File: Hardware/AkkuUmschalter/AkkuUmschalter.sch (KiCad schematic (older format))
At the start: 5 parts

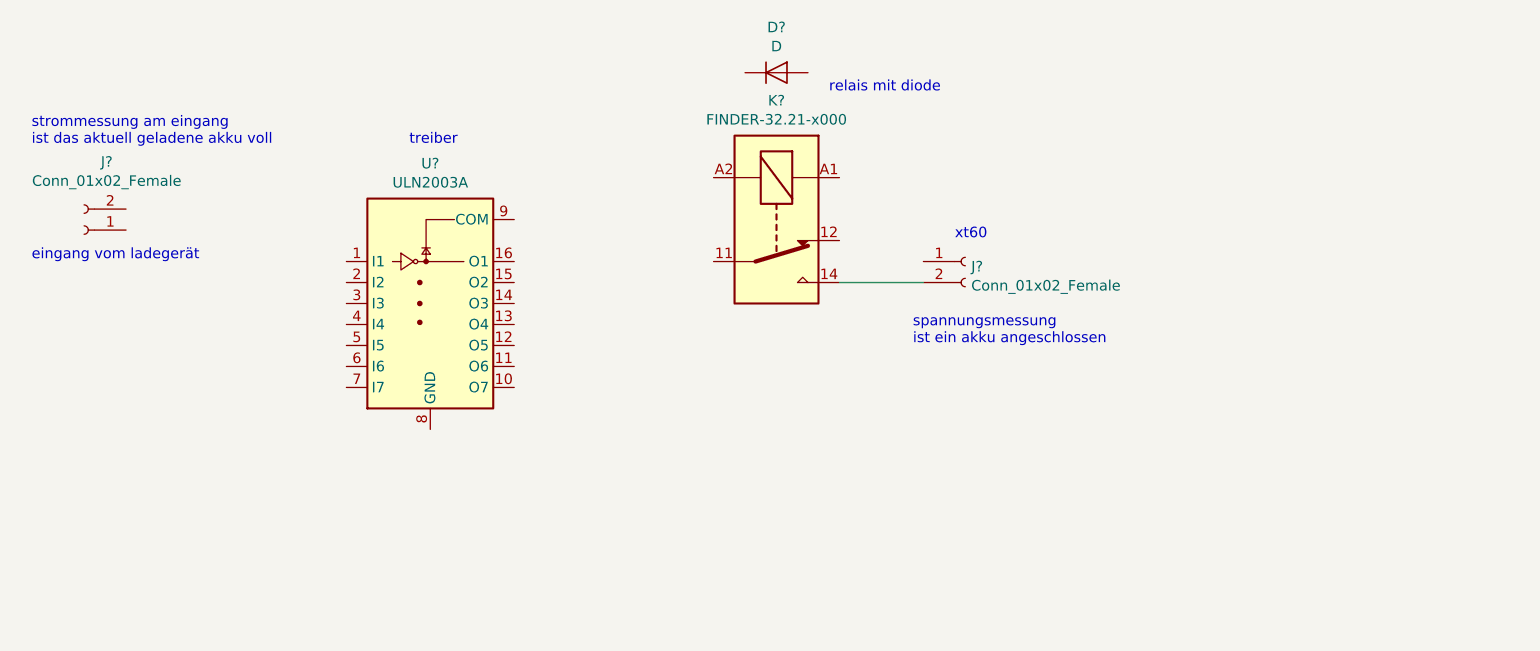
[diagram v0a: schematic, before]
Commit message: progress and voltage sensing
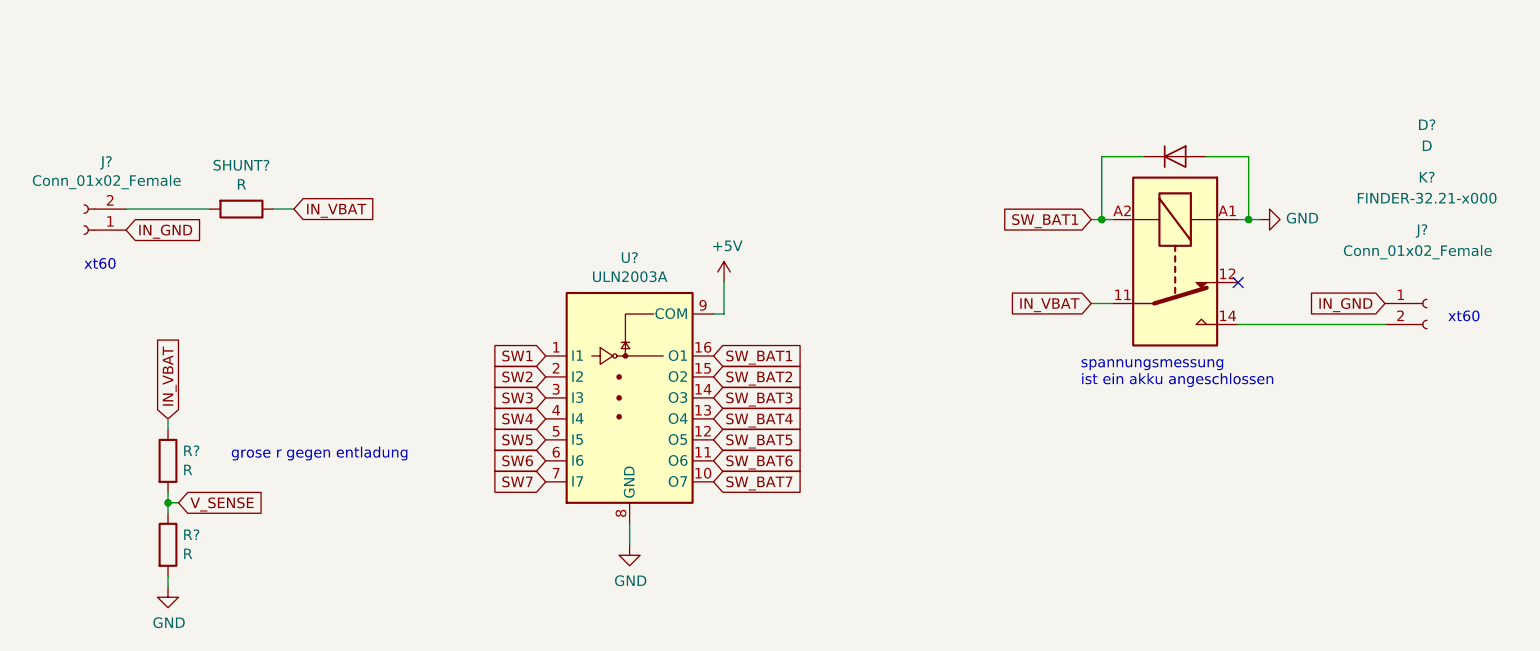
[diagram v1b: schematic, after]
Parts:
- added R? (x2), SHUNT?: R, symbol Device:R
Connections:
- net IN_VBAT: now reaches K?.11
- net IN_VBAT: now also R?.1, SHUNT?.1
- net GND: now reaches K?.A1
- net GND: now also D?.2 (A), U?.8 (GND), R?.2
- net SW_BAT1: now reaches K?.A2
- net SW_BAT1: now also D?.1 (K), U?.16 (O1)
- net IN_GND: now reaches J?.1 (Pin_1)
- net IN_GND: now also J?.1 (Pin_1)
- net SW1: now reaches U?.1 (I1)
- net SW_BAT7: now reaches U?.10 (O7)
- net SW_BAT6: now reaches U?.11 (O6)
- net SW_BAT5: now reaches U?.12 (O5)
- net SW_BAT4: now reaches U?.13 (O4)
- net SW_BAT3: now reaches U?.14 (O3)
- net SW_BAT2: now reaches U?.15 (O2)
- net SW2: now reaches U?.2 (I2)
- net SW3: now reaches U?.3 (I3)
- net SW4: now reaches U?.4 (I4)
- net SW5: now reaches U?.5 (I5)
- net SW6: now reaches U?.6 (I6)
- net SW7: now reaches U?.7 (I7)
- net +5V: now reaches U?.9 (COM)
- net at J?.2 (Pin_2): now also SHUNT?.2
- new net V_SENSE: R?.1, R?.2
- no-connect marks 0 -> 1
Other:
- note added: "grose r gegen entladung"
- note removed: "eingang vom ladegerät"
- note removed: "relais mit diode"
- note removed: "strommessung am eingang\nist das aktuell geladene akku voll"
- note removed: "treiber"
- moved on the sheet: D?, J?, K?, U?
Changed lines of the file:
@@
 L Relay:FINDER-32.21-x000 K?
 U 1 1 5E258ADA
-P 4300 1700
-F 0 "K?" V 3733 1700 50  0000 C CNN
-F 1 "FINDER-32.21-x000" V 3824 1700 50  0000 C CNN
-F 2 "" H 5570 1670 50  0001 C CNN
-F 3 "https://gfinder.findernet.com/assets/Series/355/S32EN.pdf" H 4300 1700 50  0001 C CNN
-	1    4300 1700
+P 6200 1900
+F 0 "K?" V 5800 3100 50  0000 C CNN
+F 1 "FINDER-32.21-x000" V 5900 3100 50  0000 C CNN
+F 2 "" H 7470 1870 50  0001 C CNN
+F 3 "https://gfinder.findernet.com/assets/Series/355/S32EN.pdf" H 6200 1900 50  0001 C CNN
+	1    6200 1900
 	0    1    1    0
 $EndComp
-$Comp
-L Connector:Conn_01x02_Female J?
-U 1 1 5E25A7F8
-P 5200 1900
-F 0 "J?" H 5228 1876 50  0000 L CNN
-F 1 "Conn_01x02_Female" H 5228 1785 50  0000 L CNN
-F 2 "" H 5200 1900 50  0001 C CNN
-F 3 "~" H 5200 1900 50  0001 C CNN
-	1    5200 1900
-	1    0    0    -1
-$EndComp
-Wire Wire Line
-	4600 2000 5000 2000
+Wire Wire Line
+	6500 2200 7200 2200
 $Comp
 L Transistor_Array:ULN2003A U?
 U 1 1 5E25DBBD
-P 2650 2100
-F 0 "U?" H 2650 2767 50  0000 C CNN
-F 1 "ULN2003A" H 2650 2676 50  0000 C CNN
-F 2 "" H 2700 1550 50  0001 L CNN
-F 3 "http://www.ti.com/lit/ds/symlink/uln2003a.pdf" H 2750 1900 50  0001 C CNN
-	1    2650 2100
+P 3600 2550
+F 0 "U?" H 3600 3217 50  0000 C CNN
+F 1 "ULN2003A" H 3600 3126 50  0000 C CNN
+F 2 "" H 3650 2000 50  0001 L CNN
+F 3 "http://www.ti.com/lit/ds/symlink/uln2003a.pdf" H 3700 2350 50  0001 C CNN
+	1    3600 2550
 	1    0    0    -1
 $EndComp
@@
 L Device:D D?
 U 1 1 5E25ED1E
-P 4300 1000
-F 0 "D?" H 4300 1216 50  0000 C CNN
-F 1 "D" H 4300 1125 50  0000 C CNN
-F 2 "" H 4300 1000 50  0001 C CNN
-F 3 "~" H 4300 1000 50  0001 C CNN
-	1    4300 1000
-	1    0    0    -1
-$EndComp
-Text Notes 5150 1800 0    50   ~ 0
+P 6200 1400
+F 0 "D?" H 7400 1550 50  0000 C CNN
+F 1 "D" H 7400 1450 50  0000 C CNN
+F 2 "" H 6200 1400 50  0001 C CNN
+F 3 "~" H 6200 1400 50  0001 C CNN
+	1    6200 1400
+	1    0    0    -1
+$EndComp
+Text Notes 7500 2200 0    50   ~ 0
 xt60
-Text Notes 2550 1350 0    50   ~ 0
-treiber
-Text Notes 4550 1100 0    50   ~ 0
-relais mit diode
-Text Notes 4950 2300 0    50   ~ 0
+Text Notes 5750 2500 0    50   ~ 0
 spannungsmessung\nist ein akku angeschlossen
-Text Notes 750  1350 0    50   ~ 0
-strommessung am eingang\nist das aktuell geladene akku voll
 $Comp
 L Connector:Conn_01x02_Female J?
@@
 	-1   0    0    1
 $EndComp
-Text Notes 750  1900 0    50   ~ 0
-eingang vom ladegerät
+$Comp
+L power:+5V #PWR?
+U 1 1 5E274D46
+P 4050 2000
+F 0 "#PWR?" H 4050 1850 50  0001 C CNN
+F 1 "+5V" H 4065 2173 50  0000 C CNN
+F 2 "" H 4050 2000 50  0001 C CNN
+F 3 "" H 4050 2000 50  0001 C CNN
+	1    4050 2000
+	1    0    0    -1
+$EndComp
+$Comp
+L power:GND #PWR?
+U 1 1 5E275841
+P 3600 3250
+F 0 "#PWR?" H 3600 3000 50  0001 C CNN
+F 1 "GND" H 3605 3077 50  0000 C CNN
+F 2 "" H 3600 3250 50  0001 C CNN
+F 3 "" H 3600 3250 50  0001 C CNN
+	1    3600 3250
+	1    0    0    -1
+$EndComp
+$Comp
+L power:GND #PWR?
+U 1 1 5E27671A
+P 6600 1700
+F 0 "#PWR?" H 6600 1450 50  0001 C CNN
+F 1 "GND" V 6605 1572 50  0000 R CNN
+F 2 "" H 6600 1700 50  0001 C CNN
+F 3 "" H 6600 1700 50  0001 C CNN
+	1    6600 1700
+	0    -1   -1   0
+$EndComp
+Wire Wire Line
+	6600 1700 6550 1700
+Wire Wire Line
+	6550 1700 6550 1400
+Wire Wire Line
+	6550 1400 6350 1400
+Connection ~ 6550 1700
+Wire Wire Line
+	6550 1700 6500 1700
+Wire Wire Line
+	6050 1400 5850 1400
+Wire Wire Line
+	5850 1400 5850 1700
+Wire Wire Line
+	5850 1700 5900 1700
+NoConn ~ 6500 2000
+Wire Wire Line
+	3600 3250 3600 3150
+Wire Wire Line
+	4000 2150 4050 2150
+Wire Wire Line
+	4050 2150 4050 2000
+Text GLabel 4000 2350 2    50   Input ~ 0
+SW_BAT1
+Text GLabel 4000 2450 2    50   Input ~ 0
+SW_BAT2
+Text GLabel 4000 2550 2    50   Input ~ 0
+SW_BAT3
+Text GLabel 4000 2650 2    50   Input ~ 0
+SW_BAT4
+Text GLabel 4000 2750 2    50   Input ~ 0
+SW_BAT5
+Text GLabel 4000 2850 2    50   Input ~ 0
+SW_BAT6
+Text GLabel 4000 2950 2    50   Input ~ 0
+SW_BAT7
+Text GLabel 5800 1700 0    50   Input ~ 0
+SW_BAT1
+Wire Wire Line
+	5850 1700 5800 1700
+Connection ~ 5850 1700
+$Comp
+L Connector:Conn_01x02_Female J?
+U 1 1 5E25A7F8
+P 7400 2100
+F 0 "J?" H 7350 2450 50  0000 L CNN
+F 1 "Conn_01x02_Female" H 7000 2350 50  0000 L CNN
+F 2 "" H 7400 2100 50  0001 C CNN
+F 3 "~" H 7400 2100 50  0001 C CNN
+	1    7400 2100
+	1    0    0    -1
+$EndComp
+$Comp
+L Device:R SHUNT?
+U 1 1 5E27EAD8
+P 1750 1650
+F 0 "SHUNT?" V 1543 1650 50  0000 C CNN
+F 1 "R" V 1634 1650 50  0000 C CNN
+F 2 "" V 1680 1650 50  0001 C CNN
+F 3 "~" H 1750 1650 50  0001 C CNN
+	1    1750 1650
+	0    1    1    0
+$EndComp
+Text Notes 1000 1950 0    50   ~ 0
+xt60
+Wire Wire Line
+	1200 1650 1600 1650
+Text GLabel 1200 1750 2    50   Input ~ 0
+IN_GND
+Text GLabel 7200 2100 0    50   Input ~ 0
+IN_GND
+Text GLabel 2000 1650 2    50   Input ~ 0
+IN_VBAT
+Wire Wire Line
+	2000 1650 1900 1650
+Text GLabel 5800 2100 0    50   Input ~ 0
+IN_VBAT
+Wire Wire Line
+	5800 2100 5900 2100
+Text GLabel 3200 2350 0    50   Input ~ 0
+SW1
+Text GLabel 3200 2450 0    50   Input ~ 0
+SW2
+Text GLabel 3200 2550 0    50   Input ~ 0
+SW3
+Text GLabel 3200 2650 0    50   Input ~ 0
+SW4
+Text GLabel 3200 2750 0    50   Input ~ 0
+SW5
+Text GLabel 3200 2850 0    50   Input ~ 0
+SW6
+Text GLabel 3200 2950 0    50   Input ~ 0
+SW7
+$Comp
+L Device:R R?
+U 1 1 5E281E20
+P 1400 2850
+F 0 "R?" H 1470 2896 50  0000 L CNN
+F 1 "R" H 1470 2805 50  0000 L CNN
+F 2 "" V 1330 2850 50  0001 C CNN
+F 3 "~" H 1400 2850 50  0001 C CNN
+	1    1400 2850
+	1    0    0    -1
+$EndComp
+$Comp
+L Device:R R?
+U 1 1 5E2827A1
+P 1400 3250
+F 0 "R?" H 1470 3296 50  0000 L CNN
+F 1 "R" H 1470 3205 50  0000 L CNN
+F 2 "" V 1330 3250 50  0001 C CNN
+F 3 "~" H 1400 3250 50  0001 C CNN
+	1    1400 3250
+	1    0    0    -1
+$EndComp
+Text GLabel 1450 3050 2    50   Input ~ 0
+V_SENSE
+Wire Wire Line
+	1450 3050 1400 3050
+Wire Wire Line
+	1400 3050 1400 3000
+Wire Wire Line
+	1400 3050 1400 3100
+Connection ~ 1400 3050
+$Comp
+L power:GND #PWR?
+U 1 1 5E2832FC
+P 1400 3450
+F 0 "#PWR?" H 1400 3200 50  0001 C CNN
+F 1 "GND" H 1405 3277 50  0000 C CNN
+F 2 "" H 1400 3450 50  0001 C CNN
+F 3 "" H 1400 3450 50  0001 C CNN
+	1    1400 3450
+	1    0    0    -1
+$EndComp
+Text GLabel 1400 2650 1    50   Input ~ 0
+IN_VBAT
+Wire Wire Line
+	1400 2700 1400 2650
+Wire Wire Line
+	1400 3400 1400 3450
+Text Notes 1700 2850 0    50   ~ 0
+grose r gegen entladung
 $EndSCHEMATC
